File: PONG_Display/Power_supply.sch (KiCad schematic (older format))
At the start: 21 parts, among them J2 Input_Supply+12V, U2 MCP16311MS, U3 LD1117S33TR_SOT223

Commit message: Zmiana
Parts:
- C4: footprint Capacitor_THT:CP_Axial_L10.0mm_D4.5mm_P15.00mm_Horizontal -> Capacitor_THT:CP_Radial_D8.0mm_P3.50mm
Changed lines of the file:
@@
 F 0 "C4" H 2818 6046 50  0000 L CNN
 F 1 "1u" H 2818 5955 50  0000 L CNN
-F 2 "Capacitor_THT:CP_Axial_L10.0mm_D4.5mm_P15.00mm_Horizontal" H 2738 5850 50  0001 C CNN
+F 2 "Capacitor_THT:CP_Radial_D8.0mm_P3.50mm" H 2738 5850 50  0001 C CNN
 F 3 "~" H 2700 6000 50  0001 C CNN
 	1    2700 6000

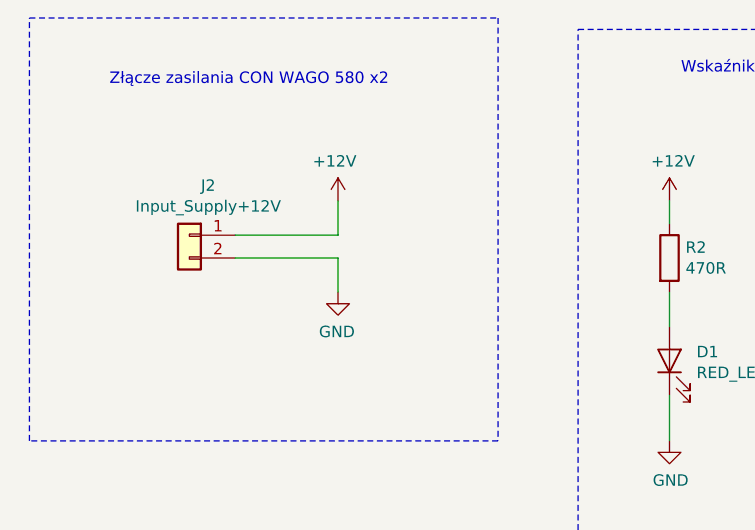
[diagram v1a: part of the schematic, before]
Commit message: zmiany
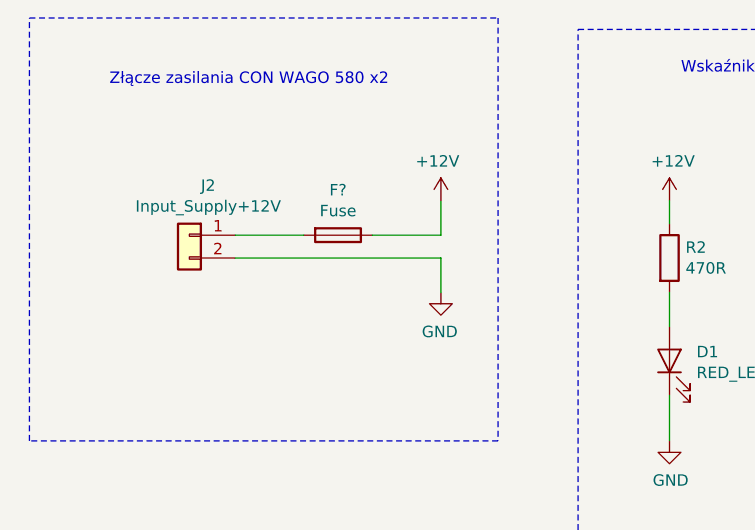
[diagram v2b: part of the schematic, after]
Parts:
- added F?: Fuse, symbol Device:Fuse
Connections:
- net +12V: now also F?.1; no longer J2.1 (Pin_1)
- new net: F?.2, J2.1 (Pin_1)
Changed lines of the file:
@@
 L power:+12V #PWR0106
 U 1 1 5E85C905
-P 2400 1600
-F 0 "#PWR0106" H 2400 1450 50  0001 C CNN
-F 1 "+12V" H 2415 1773 50  0000 C CNN
-F 2 "" H 2400 1600 50  0001 C CNN
-F 3 "" H 2400 1600 50  0001 C CNN
-	1    2400 1600
+P 2850 1600
+F 0 "#PWR0106" H 2850 1450 50  0001 C CNN
+F 1 "+12V" H 2865 1773 50  0000 C CNN
+F 2 "" H 2850 1600 50  0001 C CNN
+F 3 "" H 2850 1600 50  0001 C CNN
+	1    2850 1600
 	-1   0    0    -1
 $EndComp
@@
 L power:GND #PWR0107
 U 1 1 5E85CD82
-P 2400 2000
-F 0 "#PWR0107" H 2400 1750 50  0001 C CNN
-F 1 "GND" H 2405 1827 50  0000 C CNN
-F 2 "" H 2400 2000 50  0001 C CNN
-F 3 "" H 2400 2000 50  0001 C CNN
-	1    2400 2000
+P 2850 2000
+F 0 "#PWR0107" H 2850 1750 50  0001 C CNN
+F 1 "GND" H 2855 1827 50  0000 C CNN
+F 2 "" H 2850 2000 50  0001 C CNN
+F 3 "" H 2850 2000 50  0001 C CNN
+	1    2850 2000
 	-1   0    0    -1
 $EndComp
 Wire Wire Line
-	2400 1600 2400 1750
-Wire Wire Line
-	2400 1750 1950 1750
-Wire Wire Line
-	2400 1850 2400 2000
-Wire Wire Line
-	2400 1850 1950 1850
+	2850 1600 2850 1750
+Wire Wire Line
+	2850 1850 2850 2000
+Wire Wire Line
+	2850 1850 1950 1850
 $Comp
 L Regulator_Linear:LD1117S33TR_SOT223 U3
@@
 	4100 5500 4200 5500
 Connection ~ 4100 5500
+$Comp
+L Device:Fuse F?
+U 1 1 5EA039B3
+P 2400 1750
+F 0 "F?" V 2203 1750 50  0000 C CNN
+F 1 "Fuse" V 2294 1750 50  0000 C CNN
+F 2 "" V 2330 1750 50  0001 C CNN
+F 3 "~" H 2400 1750 50  0001 C CNN
+	1    2400 1750
+	0    1    1    0
+$EndComp
+Wire Wire Line
+	2550 1750 2850 1750
+Wire Wire Line
+	2250 1750 1950 1750
 $EndSCHEMATC
